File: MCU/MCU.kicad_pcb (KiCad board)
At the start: 2 copper layers, 105.5 x 79 mm, 78 parts, among them J2 Conn_01x02, J3 Conn_01x02, J4 Conn_01x02, J5 Conn_01x02, J6 Conn_01x04, U1 Nucleo_L432KC, U3 HHG1D-1, U4 AMC3302QDWERQ1, U5 HHG1D-1, U6 AMC3302QDWERQ1, U7 HHG1D-1, U8 AMC3302QDWERQ1, U9 MAX31865xAP

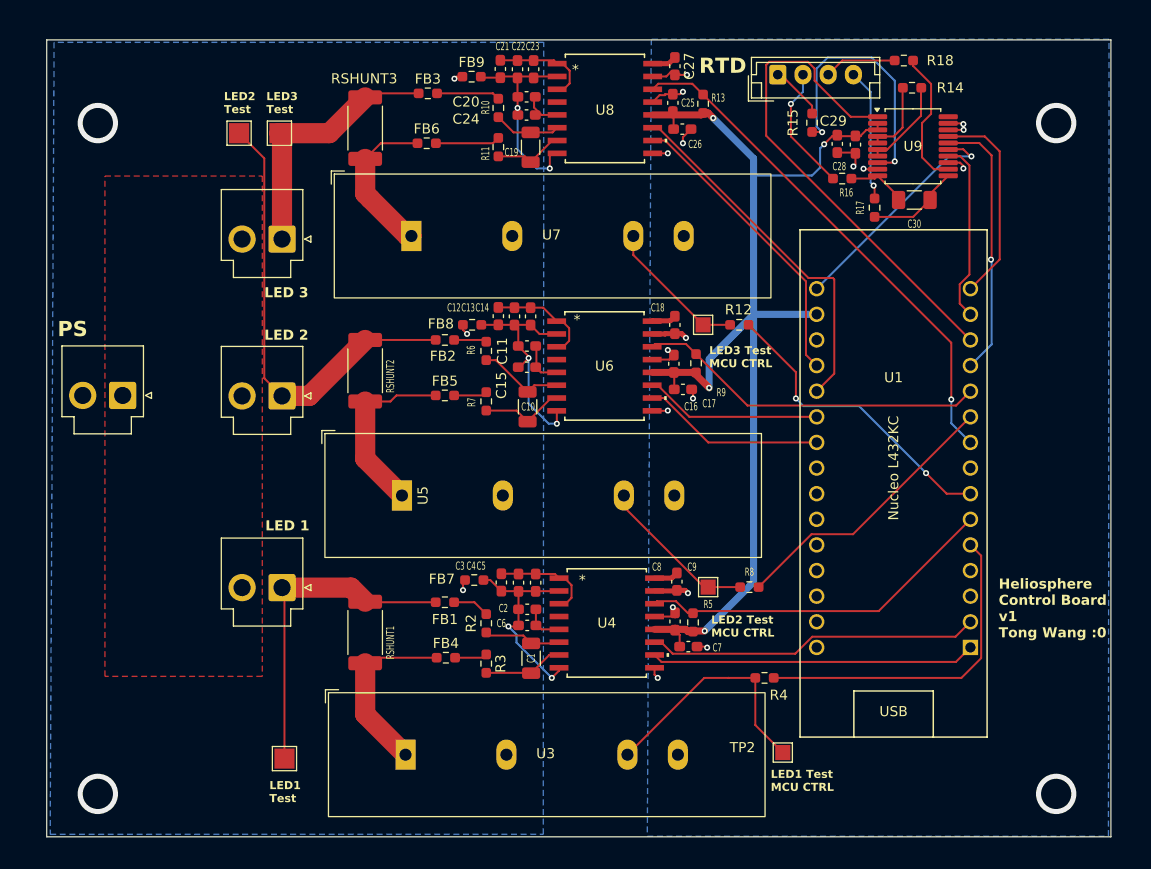
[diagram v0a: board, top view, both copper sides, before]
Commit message: silkscreen, edge cuts, other stuff fixes
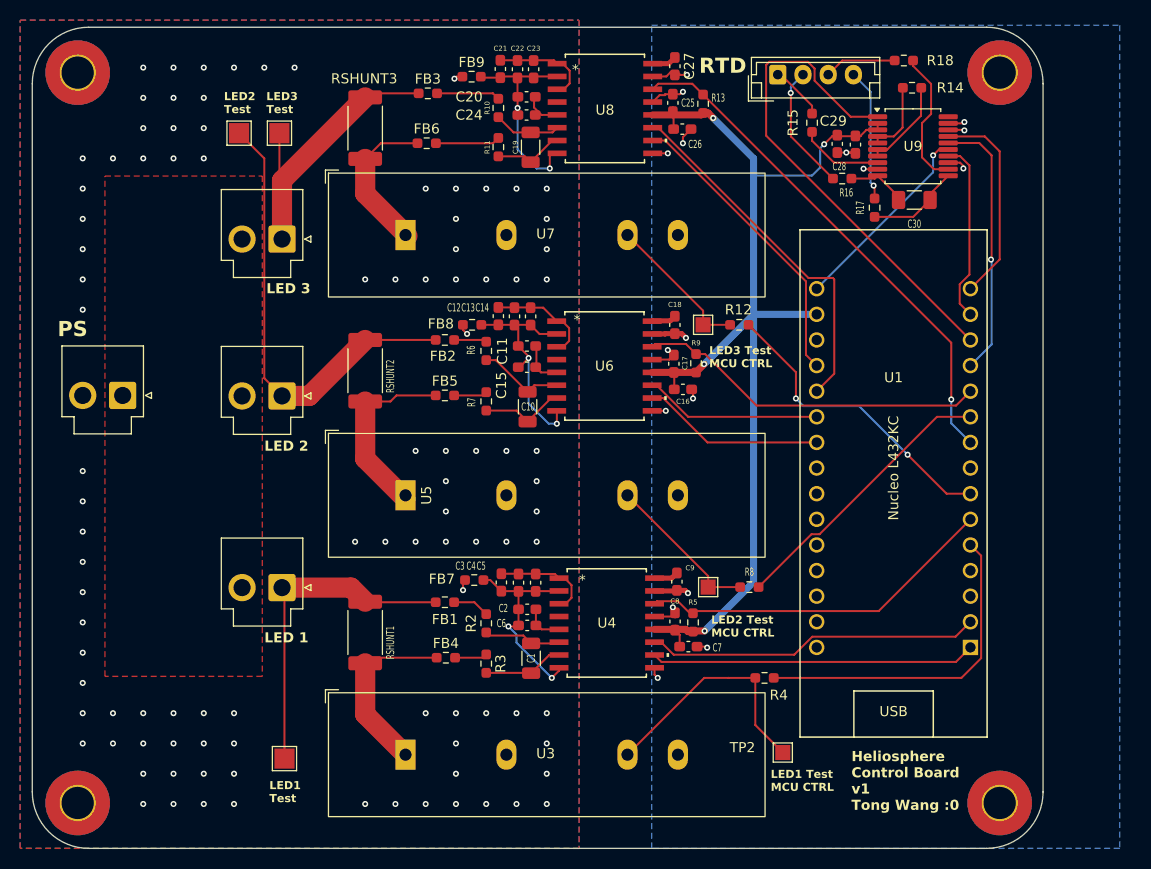
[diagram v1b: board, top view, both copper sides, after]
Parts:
- added H1: MountingHole_Pad, MountingHole:MountingHole_3.2mm_M3_Pad_TopBottom, F.Cu at (95.5, 54.5)
- added H2: MountingHole_Pad, MountingHole:MountingHole_3.2mm_M3_Pad_TopBottom, F.Cu at (95.5, 126.9)
- added H3: MountingHole_Pad, MountingHole:MountingHole_3.2mm_M3_Pad_TopBottom, F.Cu at (186.9, 54.5)
- added H4: MountingHole_Pad, MountingHole:MountingHole_3.2mm_M3_Pad_TopBottom, F.Cu at (186.9, 126.9)
- moved U7 0.59 mm to (128.0, 70.6)
- moved U5 0.35 mm to (128.0, 96.4)
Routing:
- net Net-(U9-FORCE+): track 26.4 -> 8.27 mm, vias 2 -> 0
- net /D13: track 23.4 -> 19.7 mm
- net +3V3: track 115.7 -> 112.8 mm
- net /LED3: track 26.0 -> 27.7 mm
- net Net-(FB5-Pad1): track 18.4 -> 18.9 mm
- net GND: track 38.8 -> 38.3 mm
- net GND1: vias 3 -> 101
- net (no net): vias 4 -> 0
- added copper zone on F.Cu, net GND1
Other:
- board size 105.5 x 79 mm -> 100.2 x 81.4 mm
